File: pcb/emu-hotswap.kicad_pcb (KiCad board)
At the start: 2 copper layers, 160.1 x 118.5 mm, 77 parts, among them J1 TRRS, SW1 SW_Push, SW10 SW_Push, SW11 SW_Push, SW12 SW_Push, SW13 SW_Push, SW14 SW_Push, SW15 SW_Push, SW16 SW_Push, SW17 SW_Push, SW18 SW_Push, SW19 SW_Push, SW2 SW_Push, SW20 SW_Push, SW21 SW_Push, SW22 SW_Push, SW23 SW_Push, SW24 SW_Push, SW25 SW_Push, SW26 SW_Push, SW27 SW_Push, SW28 SW_Push, SW29 SW_Push, SW3 SW_Push, SW30 SW_Push, SW31 SW_Push, SW4 SW_Push, SW5 SW_Push, SW6 SW_Push, SW7 SW_Push, SW8 SW_Push, SW9 SW_Push, U1 ProMicro

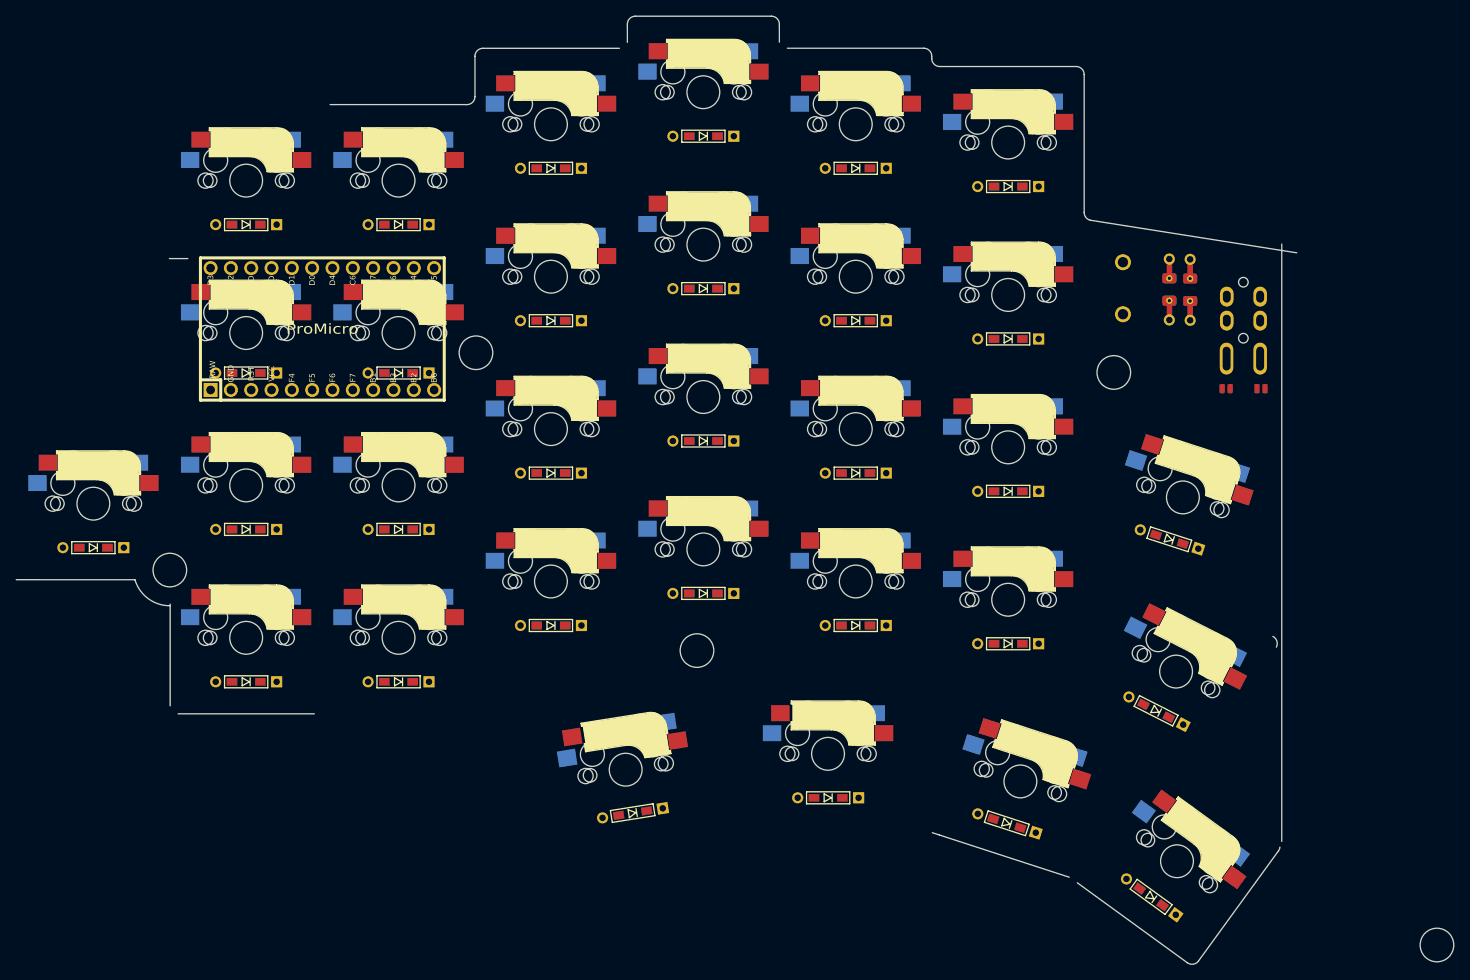
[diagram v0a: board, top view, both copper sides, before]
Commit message: Roughly cut edges, fixed footprints on the scheme.
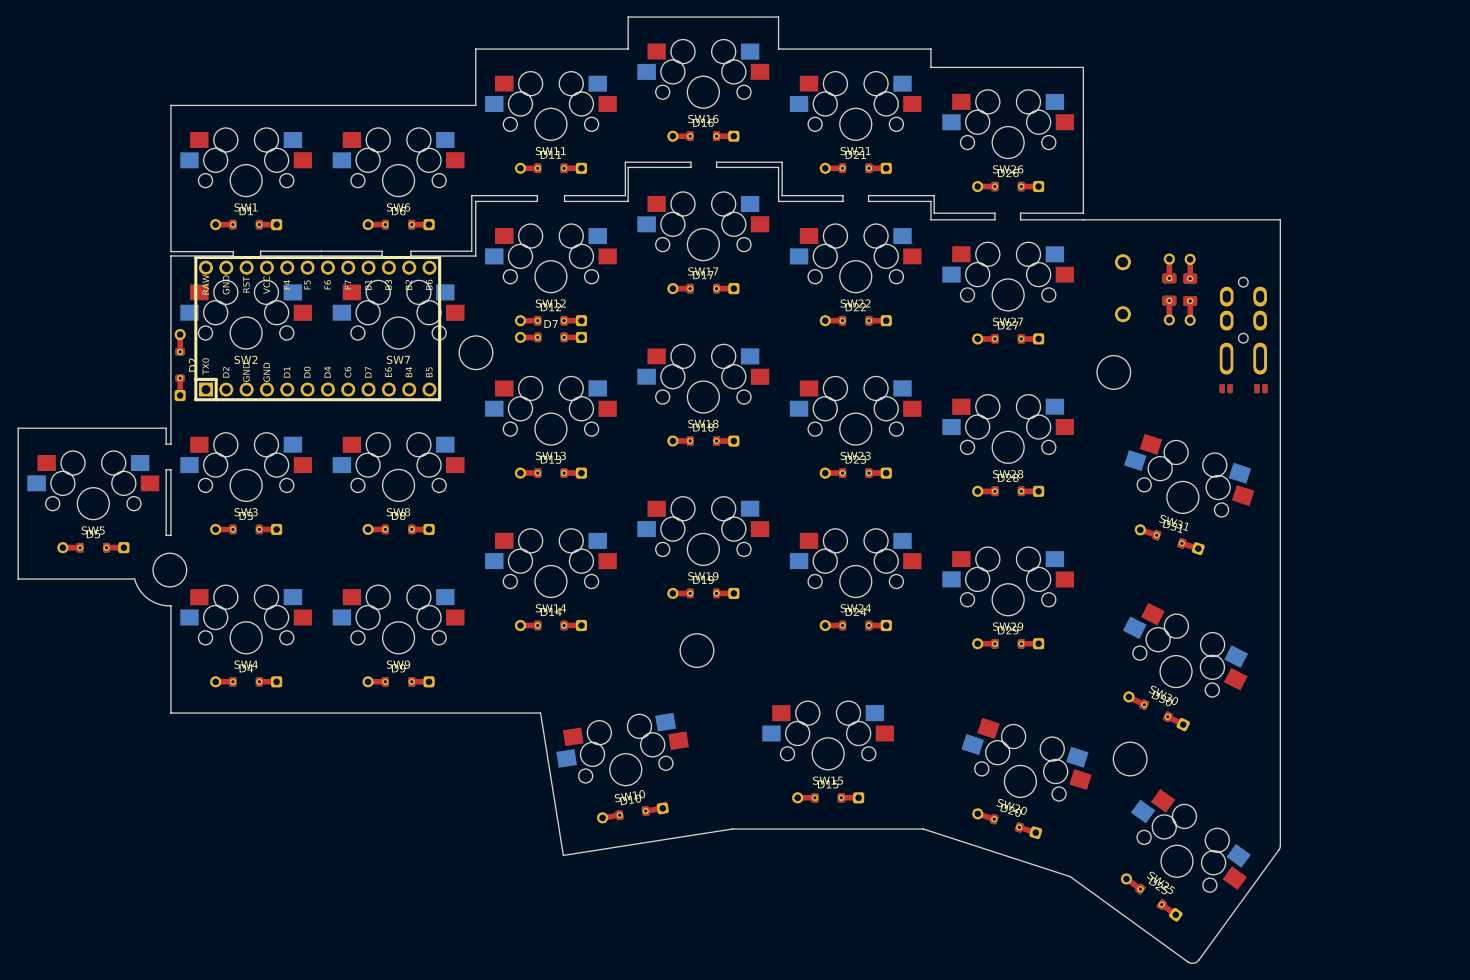
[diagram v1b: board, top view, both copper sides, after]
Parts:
- removed the D10 at (220.4, 95.8)
- removed the D10 at (153.3, 130.1)
- removed G***: LOGO, used_footprints:emu-logo
- removed the SW10 at (152.5, 124.6)
- removed the SW10 at (222.1, 90.6)
- added D10: 1N4148, used_footprints:Diode_Hybrid_SOD-123, F.Cu at (153.3, 130.1)
- added D31: 1N4148, used_footprints:Diode_Hybrid_SOD-123, F.Cu at (220.4, 95.8)
- added SW10: SW_Push, used_footprints:Switch_Mx_Hotswap_1u, F.Cu at (152.5, 124.6)
- added SW31: SW_Push, used_footprints:Switch_Mx_Hotswap_1u, F.Cu at (222.1, 90.6)
- D1, D11, D12, D13, D14, D15, D16, D17, D18, D19, D2, D20, D21, D22, D23, D24, D25, D26, D27, D28, D29, D3, D30, D4, D5, D6, D7, D8, D9: footprint used_footprints:D3_TH_SMD -> used_footprints:Diode_Hybrid_SOD-123
- SW1, SW11, SW12, SW13, SW14, SW16, SW17, SW18, SW19, SW2, SW20, SW21, SW22, SW23, SW24, SW25, SW26, SW27, SW28, SW29, SW3, SW30, SW4, SW5, SW6, SW7, SW8, SW9: footprint used_footprints:CherryMX_MidHeight_Hotswap_1u -> used_footprints:Switch_Mx_Hotswap_1u
- SW15: footprint used_footprints:CherryMX_MidHeight_Hotswap_1.25u -> used_footprints:Switch_Mx_Hotswap_1u
- U1: footprint used_footprints:Pro_Micro -> used_footprints:ArduinoProMicro
- moved HM1 44.8 mm to (215.5, 123.3)
- moved D7 19.6 mm to (143.1, 70.6)
- moved D2 8.31 mm to (96.8, 74.0), turned to 90 degrees
- moved U1 0.95 mm to (114.0, 69.5), turned to 0 degrees
- renumbered SW31 to SW32
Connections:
- U1 pad 17: (no net) -> /rowF
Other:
- board size 160.1 x 118.5 mm -> 157.8 x 118.3 mm
